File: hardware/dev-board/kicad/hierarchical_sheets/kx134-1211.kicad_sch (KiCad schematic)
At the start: 14 parts, among them U2 KX134-1211

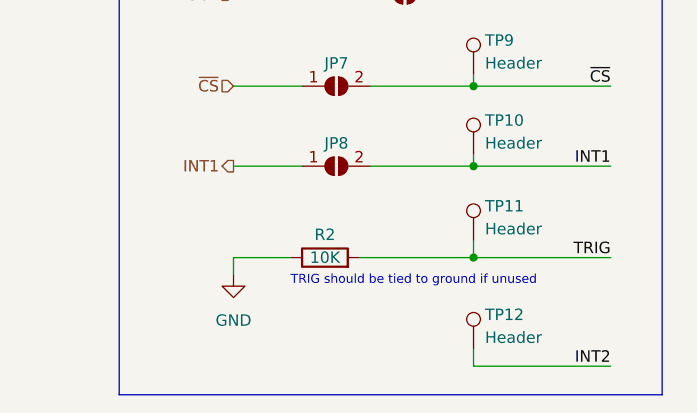
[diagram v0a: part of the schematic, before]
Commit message: rf is hard
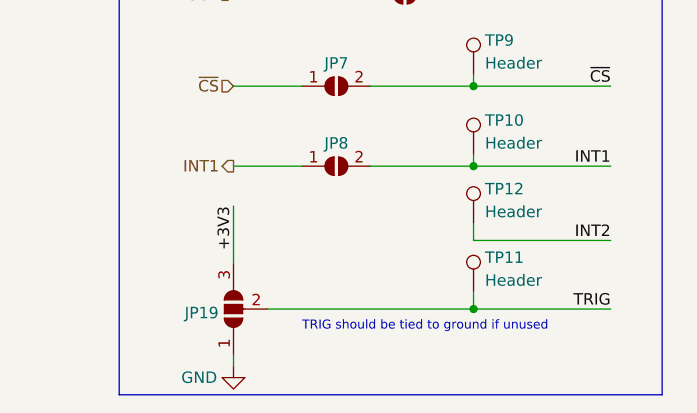
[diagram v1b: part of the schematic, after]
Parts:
- removed R2: 10K, symbol Device:R
- added JP19: SolderJumper_3_Open, Jumper:SolderJumper-3_P1.3mm_Open_RoundedPad1.0x1.5mm, symbol Jumper:SolderJumper_3_Open
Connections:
- net +3V3: now also JP19.3 (B)
- net GND: now also JP19.1 (A)
- net TRIG: now also JP19.2 (C)
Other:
- moved on the sheet: TP12
